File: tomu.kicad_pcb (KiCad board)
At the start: 2 copper layers, 13 x 11 mm, 16 parts, among them P1 DEBUG, P3 USB-PCB, U1 MKL27Z256VFM4, U2 ateccXXXa

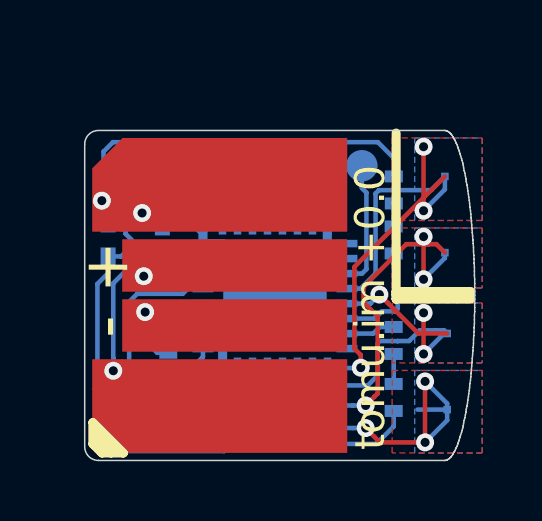
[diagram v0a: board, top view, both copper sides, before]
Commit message: Adding slot.
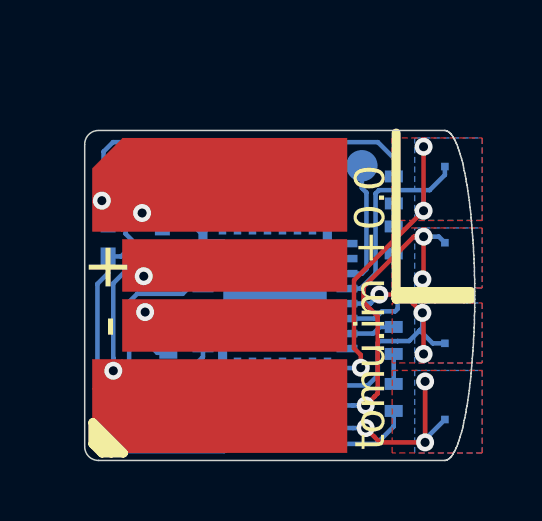
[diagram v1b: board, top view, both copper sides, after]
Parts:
- added REF**: Measurement_Point_Round-TH_Small, usb-pcb:slot, F.Cu at (29.1, 23.5)
- moved W2 0.34 mm to (29.0, 25.1)
- moved W1 0.33 mm to (29.0, 19.2)
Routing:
- net /CAP1B: track 11.7 -> 9.14 mm
- net /CAP1A: track 13.3 -> 11.4 mm
- net /CAP0A: track 18.8 -> 16.9 mm
- net /CAP0B: track 13.6 -> 12.3 mm
